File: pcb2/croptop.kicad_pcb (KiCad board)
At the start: 4 copper layers, 190.1 x 107.2 mm, 403 parts, among them J1 TSM-106-01-L-SV, J10 1702474, J11 1702474, J12 1702474, J13 1702474, J14 1702474, J15 TSM-112-01-L-DV, J16 DM3D-SF, J2 0473460001, J3 87583-2010BLF, J4 TSM-102-01-L-DV, J5 686104183422, J6 62684-402100ALF, J7 1702474, J8 1702474, J9 1702474, Q1 BSS138, Q2 BSS84, Q3 Q2319ADS-T1-GE3, Q4 BSS138, Q5 BSS138, Q6 BSS138, SW1 SW_Push, SW2 SW_Push, SW3 SW_Push, SW4 SW_Push, U1 PIC32MX795F512L, U10 TPD4E1U06DBV, U11 TPD4E1U06DBV, U12 TPD4E1U06DBV, U13 TPD4E1U06DBV, U14 TPD4E1U06DBV, U15 TPD4E1U06DBV, U16 TPD4E1U06DBV, U17 TPD4E1U06DBV, U18 74HCT125D653, U19 AP22802AW5, U2 REG71055DDC, U20 AD7799, U21 AP22802AW5, U22 TPD4E1U06DBV, U23 AP22802AW5, U24 TPD4E1U06DBV, U25 TPD4E1U06DBV, U26 TPD4E1U06DBV, U27 DRV8872, U28 DRV8825, U29 AP22802AW5, U3 AP22802AW5, U30 TPD4E1U06DBV, U31 TPD4E1U06DBV, U32 AP22802AW5, U33 AP22802AW5, U34 TPD4E1U06DBV, U35 TPD4E1U06DBV, U36 AP22802AW5, U37 TPD4E1U06DBV, U38 TPD4E1U06DBV, U39 LIS3DSHTR, U4 TPS61169DCK, U40 CAM-M8C-0, U41 Si7006-A20, U5 TPS62131RGT, U6 TPS70950DBV, U7 TPD4E1U06DBV, U8 TPD4E1U06DBV, U9 FT812Q, Y1 ABLS-8.000MHZ-B4-T, Y2 ABLS-12.000MHZ-B2-T

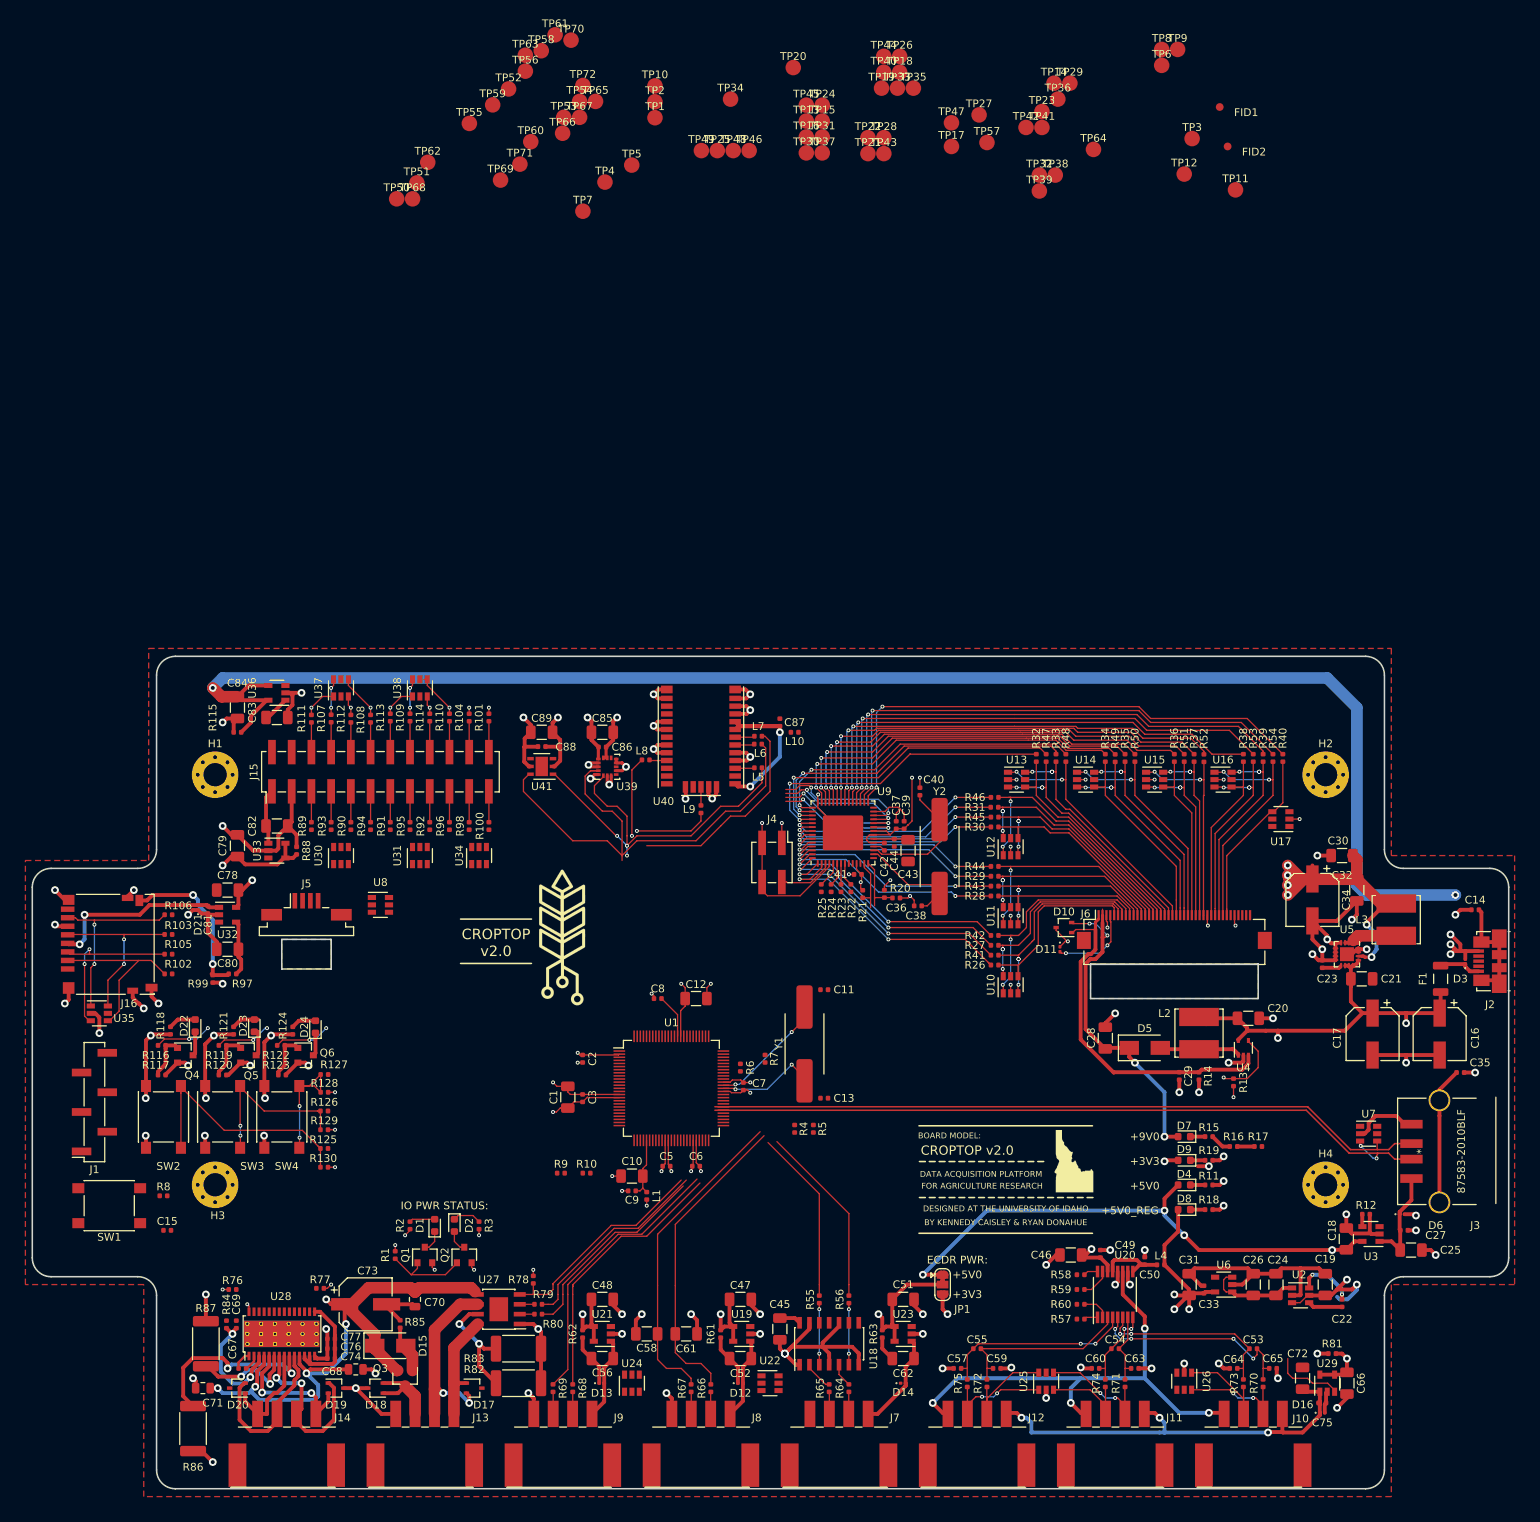
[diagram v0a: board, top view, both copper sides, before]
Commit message: Finished PCB
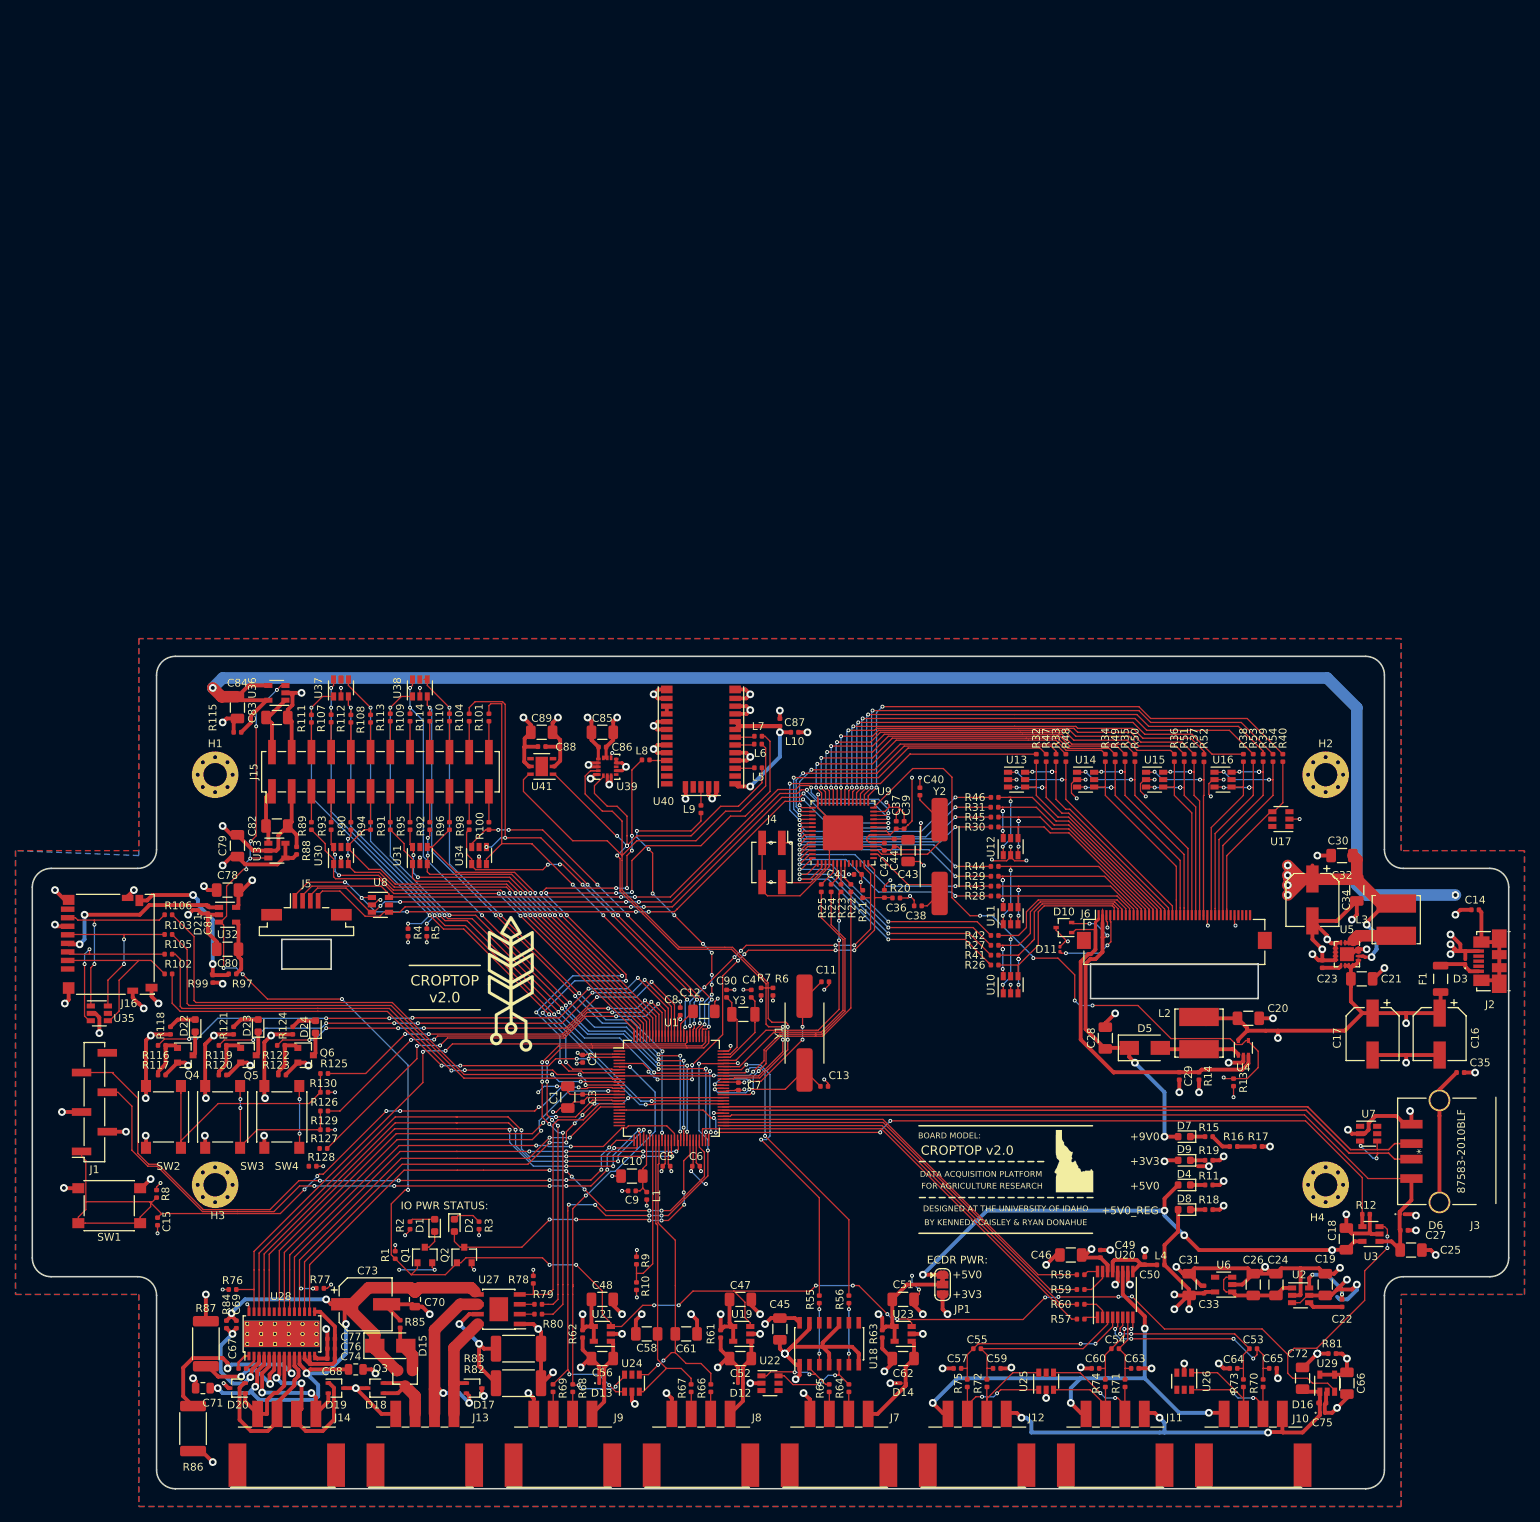
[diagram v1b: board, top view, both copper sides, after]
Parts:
- removed FID1, FID2: Fiducial, Fiducial:Fiducial_1mm_Dia_2.54mm_Outer_CopperTop
- removed TP1, TP10, TP11, TP12, TP13, TP14, TP15, TP16, TP17, TP18, TP19, TP2, TP20, TP21, TP22, TP23, TP24, TP25, TP26, TP27, TP28, TP29, TP3, TP30, TP31, TP32, TP33, TP34, TP35, TP36, TP37, TP38, TP39, TP4, TP40, TP41, TP42, TP43, TP44, TP45, TP46, TP47, TP48, TP49, TP5, TP50, TP51, TP52, TP53, TP54, TP55, TP56, TP57, TP58, TP59, TP6, TP60, TP61, TP62, TP63, TP64, TP65, TP66, TP67, TP68, TP69, TP7, TP70, TP71, TP72, TP8, TP9: TestPoint, croptop:TestPoint
- added C4: 12.5p, Capacitor_SMD:C_0402_1005Metric, F.Cu at (144.9, 98.4)
- added C90: 12.5p, Capacitor_SMD:C_0402_1005Metric, F.Cu at (141.7, 98.4)
- added Y3: ABS07-32.768KHZ-1-T, croptop:ABLS_SEC, F.Cu at (143.9, 101.1)
- moved R4 55.8 mm to (100.7, 90.6), turned to 90 degrees
- moved R5 55.8 mm to (103.1, 90.6), turned to 90 degrees
- moved R10 15.9 mm to (130.1, 136.1), turned to 270 degrees
- moved R9 14.9 mm to (130.1, 132.8), turned to 270 degrees
- moved R6 10.6 mm to (147.7, 98.2), turned to 90 degrees
- moved R125 9.65 mm to (89.9, 108.7)
- moved R130 9.65 mm to (89.9, 111.1)
- moved R128 9.65 mm to (88.4, 120.7)
- moved R127 9.53 mm to (89.8, 118.4)
- moved G*** 8.90 mm to (113.8, 97.9)
- moved R7 8.65 mm to (146.2, 98.2), turned to 90 degrees
- moved C8 3.34 mm to (135.8, 100.7), turned to 90 degrees
- moved C12 1.94 mm to (138.8, 100.7)
- moved C15 1.69 mm to (68.5, 127.8), turned to 270 degrees
- moved C13 1.52 mm to (154.3, 110.4)
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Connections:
- U1 pad 1: ~ADI_CS -> Net-(U1-Pad1)
- U1 pad 10: GPU_SCLK -> SD_SCLK
- U1 pad 11: GPU_MISO -> SD_MISO
- U1 pad 12: GPU_MOSI -> SD_MOSI
- U1 pad 33: POTEN_ADC_1 -> POTEN_ADC_2
- U1 pad 34: POTEN_ADC_2 -> POTEN_ADC_1
- U1 pad 4: ~GPU_CS -> Net-(U1-Pad4)
- U1 pad 44: Net-(U1-Pad44) -> Net-(D2-Pad2)
- U1 pad 48: SD_SCLK -> ADI_SCLK
- U1 pad 51: Net-(U1-Pad51) -> ~ADI_CS
- U1 pad 52: SD_MISO -> ADI_MISO
- U1 pad 53: SD_MOSI -> ADI_MOSI
- U1 pad 61: Net-(U1-Pad61) -> ~GPU_CS
- U1 pad 70: ADI_SCLK -> GPU_SCLK
- U1 pad 72: ADI_MOSI -> GPU_MOSI
- U1 pad 74: ~PWR_FAULT -> Net-(C90-Pad1)
- U1 pad 9: ADI_MISO -> GPU_MISO
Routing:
- net ~PWR_FAULT: track 20.4 -> 271.3 mm, vias 0 -> 23
- net DGND: track 465.5 -> 581.8 mm, vias 119 -> 172
- net USB_PWR_EN: track 1.60 -> 107.9 mm, vias 0 -> 4
- net PICKIT_MCLR: track 0.00 -> 99.3 mm, vias 0 -> 6
- net USB_PWR_SENSE: track 13.0 -> 105.1 mm
- net PICKIT_PGEC: track 0.00 -> 87.5 mm, vias 0 -> 6
- net PMOD_SCL: track 4.39 -> 89.3 mm, vias 1 -> 5
- net PMOD_TX: track 2.51 -> 86.4 mm, vias 1 -> 6
- net PICKIT_PGED: track 0.00 -> 83.4 mm, vias 0 -> 6
- net PMOD_RX: track 5.76 -> 87.9 mm, vias 1 -> 6
- net PMOD_SDA: track 4.68 -> 86.2 mm, vias 2 -> 6
- net ~STEP_HOME: track 0.00 -> 80.1 mm, vias 0 -> 2
- net PMOD_ADC_4: track 4.24 -> 82.6 mm, vias 1 -> 6
- net GPU_PWM: track 9.11 -> 85.5 mm, vias 1 -> 5
- net PMOD_ADC_3: track 4.56 -> 79.1 mm, vias 2 -> 7
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- added copper zone on B.Cu, net DGND
